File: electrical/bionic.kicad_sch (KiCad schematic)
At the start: 22 parts, among them J1 GPIO, U1 CAT24C256

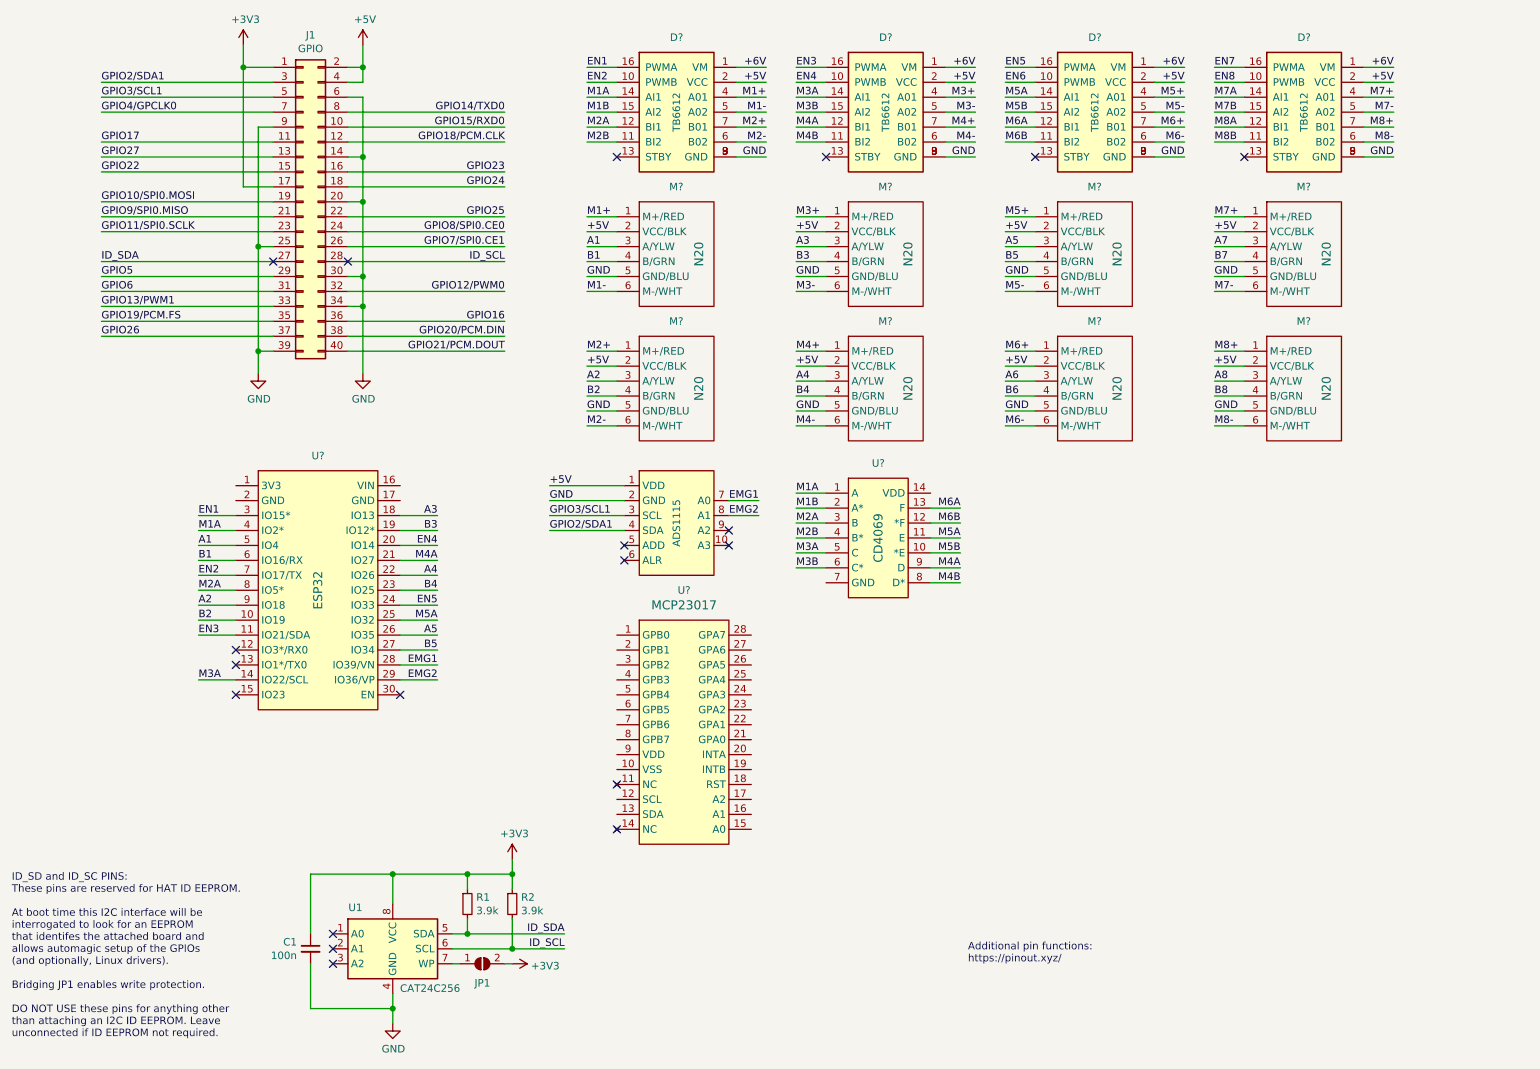
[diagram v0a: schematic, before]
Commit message: add(electrical/symbol): Updated Components
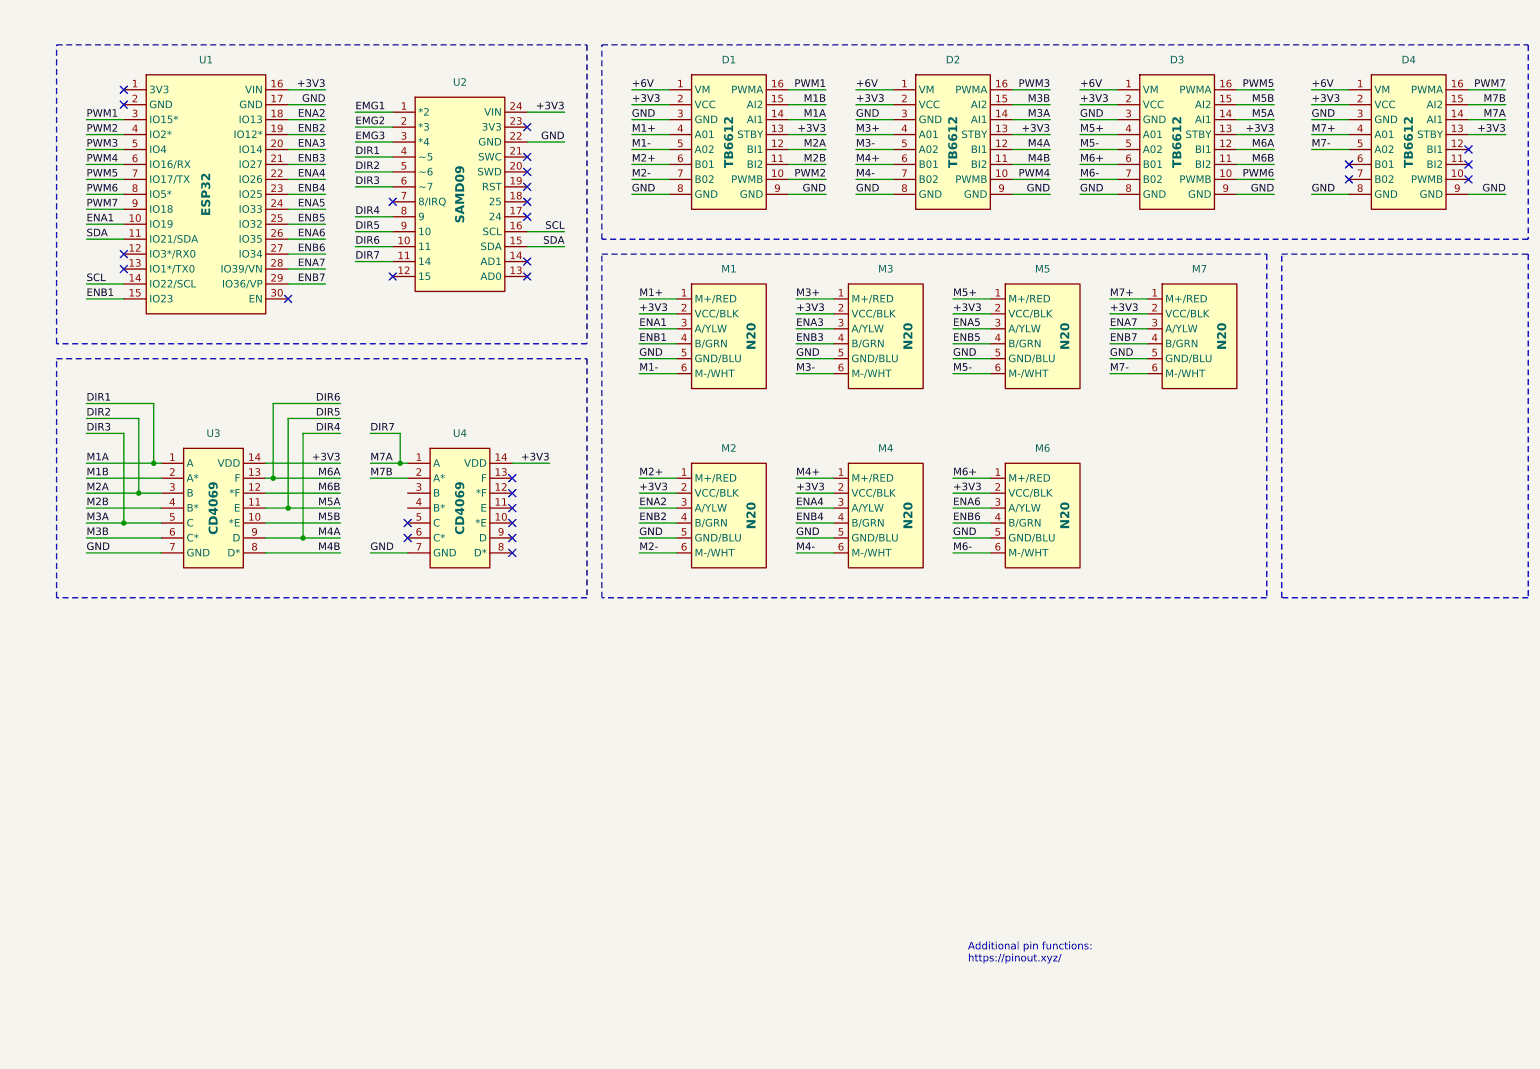
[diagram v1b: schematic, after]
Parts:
- removed C1: 100n, symbol Device:C_Small
- removed D? (x4): TB6612, symbol Motor_Driver:TB6612_DC_Driver
- removed J1: GPIO, Connector_PinSocket_2.54mm:PinSocket_2x20_P2.54mm_Vertical, symbol Connector_Generic:Conn_02x20_Odd_Even
- removed JP1: ID_WP, symbol Jumper:SolderJumper_2_Open
- removed M? (x8): N20, symbol bionic:N20_EN
- removed R1, R2: 3.9k, symbol Device:R_Small
- removed U1: CAT24C256, symbol Memory_EEPROM:CAT24C256
- removed U?: MCP23017, symbol bionic:MCP23017
- removed U?: CD4069, symbol bionic:CD4069
- removed U?: ESP32, symbol bionic:ESP32
- removed U?: ADS1115, symbol bionic:ADS1115
- added D1, D2, D3, D4: TB6612, symbol bionic:TB6612
- added M1, M2, M3, M4, M5, M6, M7: N20, symbol bionic:N20_EN
- added U1: ESP32, symbol bionic:ESP32
- added U2: SAMD09, symbol bionic:SAMD09
- added U3, U4: CD4069, symbol bionic:CD4069
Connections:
- net +3V3: now also D1.13 (STBY), D1.2 (VCC), D2.13 (STBY), D2.2 (VCC), D3.13 (STBY), D3.2 (VCC), D4.13 (STBY), D4.2 (VCC), M1.2 (VCC/BLK), M2.2 (VCC/BLK), M3.2 (VCC/BLK), M4.2 (VCC/BLK), M5.2 (VCC/BLK), M6.2 (VCC/BLK), M7.2 (VCC/BLK), U1.16 (VIN), U2.24 (VIN), U3.14 (VDD), U4.14 (VDD)
- net +6V: now also D1.1 (VM), D2.1 (VM), D3.1 (VM), D4.1 (VM)
- net EMG1: now also U2.1 (*2)
- net EMG2: now also U2.2 (*3)
- net GND: now also D1.3 (GND), D1.8 (GND), D1.9 (GND), D2.3 (GND), D2.8 (GND), D2.9 (GND), D3.3 (GND), D3.8 (GND), D3.9 (GND), D4.3 (GND), D4.8 (GND), D4.9 (GND), M1.5 (GND/BLU), M2.5 (GND/BLU), M3.5 (GND/BLU), M4.5 (GND/BLU), M5.5 (GND/BLU), M6.5 (GND/BLU), M7.5 (GND/BLU), U1.17 (GND), U2.22 (GND), U3.7 (GND), U4.7 (GND)
- net M1+: now also D1.4 (A01), M1.1 (M+/RED)
- net M1-: now also D1.5 (A02), M1.6 (M-/WHT)
- net M1B: now also D1.15 (AI2), U3.2 (A*)
- net M2+: now also D1.6 (B01), M2.1 (M+/RED)
- net M2-: now also D1.7 (B02), M2.6 (M-/WHT)
- net M2B: now also D1.11 (BI2), U3.4 (B*)
- net M3+: now also D2.4 (A01), M3.1 (M+/RED)
- net M3-: now also D2.5 (A02), M3.6 (M-/WHT)
- net M3B: now also D2.15 (AI2), U3.6 (C*)
- net M4+: now also D2.6 (B01), M4.1 (M+/RED)
- net M4-: now also D2.7 (B02), M4.6 (M-/WHT)
- net M4B: now also D2.11 (BI2), U3.8 (D*)
- net M5+: now also D3.4 (A01), M5.1 (M+/RED)
- net M5-: now also D3.5 (A02), M5.6 (M-/WHT)
- net M5B: now also D3.15 (AI2), U3.10 (*E)
- net M6+: now also D3.6 (B01), M6.1 (M+/RED)
- net M6-: now also D3.7 (B02), M6.6 (M-/WHT)
- net M6B: now also D3.11 (BI2), U3.12 (*F)
- net M7+: now also D4.4 (A01), M7.1 (M+/RED)
- net M7-: now also D4.5 (A02), M7.6 (M-/WHT)
- net M7B: now also D4.15 (AI2), U4.2 (A*)
- new net DIR1: D1.14 (AI1), U2.4 (~5), U3.1 (A)
- new net DIR2: D1.12 (BI1), U2.5 (~6), U3.3 (B)
- new net DIR3: D2.14 (AI1), U2.6 (~7), U3.5 (C)
- new net DIR4: D2.12 (BI1), U2.8 (9), U3.9 (D)
- new net DIR5: D3.14 (AI1), U2.9 (10), U3.11 (E)
- new net DIR6: D3.12 (BI1), U2.10 (11), U3.13 (F)
- new net DIR7: D4.14 (AI1), U2.11 (14), U4.1 (A)
- new net EMG3: U2.3 (*4)
- new net ENA1: M1.3 (A/YLW), U1.10 (IO19)
- new net ENA2: M2.3 (A/YLW), U1.18 (IO13)
- new net ENA3: M3.3 (A/YLW), U1.20 (IO14)
- new net ENA4: M4.3 (A/YLW), U1.22 (IO26)
- new net ENA5: M5.3 (A/YLW), U1.24 (IO33)
- new net ENA6: M6.3 (A/YLW), U1.26 (IO35)
- new net ENA7: M7.3 (A/YLW), U1.28 (IO39/VN)
- new net ENB1: M1.4 (B/GRN), U1.15 (IO23)
- new net ENB2: M2.4 (B/GRN), U1.19 (IO12*)
- new net ENB3: M3.4 (B/GRN), U1.21 (IO27)
- new net ENB4: M4.4 (B/GRN), U1.23 (IO25)
- new net ENB5: M5.4 (B/GRN), U1.25 (IO32)
- new net ENB6: M6.4 (B/GRN), U1.27 (IO34)
- new net ENB7: M7.4 (B/GRN), U1.29 (IO36/VP)
- new net PWM1: D1.16 (PWMA), U1.3 (IO15*)
- new net PWM2: D1.10 (PWMB), U1.4 (IO2*)
- new net PWM3: D2.16 (PWMA), U1.5 (IO4)
- new net PWM4: D2.10 (PWMB), U1.6 (IO16/RX)
- new net PWM5: D3.16 (PWMA), U1.7 (IO17/TX)
- new net PWM6: D3.10 (PWMB), U1.8 (IO5*)
- new net PWM7: D4.16 (PWMA), U1.9 (IO18)
- new net SCL: U1.14 (IO22/SCL), U2.16 (SCL)
- new net SDA: U1.11 (IO21/SDA), U2.15 (SDA)
- no-connect marks 19 -> 28
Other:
- note removed: "ID_SD and ID_SC PINS: These pins are reserved for HAT ID EEPROM. At boot time this I2C interface will be interrogated to look for an EEPROM that identifes the attached board and allows automagic setup of the GPIOs (and optionally, Linux drivers). Bridging JP1 enables write protection. DO NOT USE these pins for anything other than attaching an I2C ID EEPROM. Leave unconnected if ID EEPROM not requ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"
